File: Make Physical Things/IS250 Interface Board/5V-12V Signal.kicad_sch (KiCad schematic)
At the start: 5 parts, among them Q10 PN2222A, Q11 PN2907A

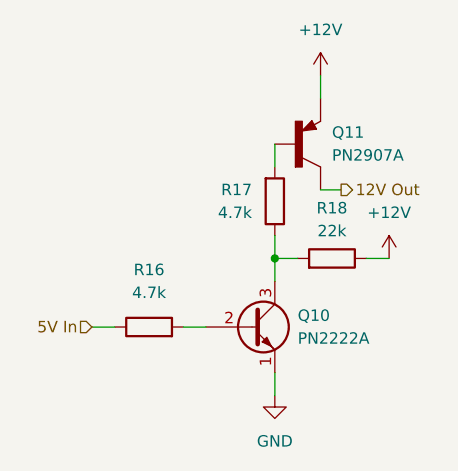
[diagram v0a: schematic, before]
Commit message: More PCB Layout
PCB laid out further, and just requires routing and silkscreen.
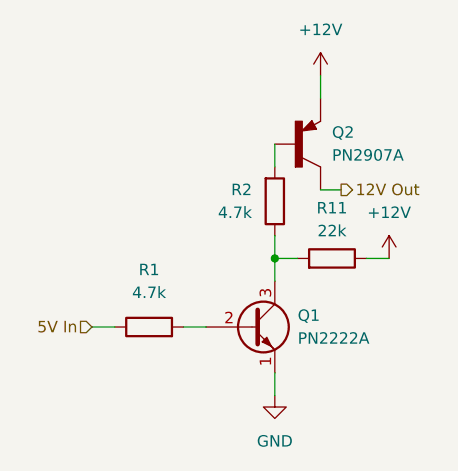
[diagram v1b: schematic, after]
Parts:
- renumbered Q10 to Q1, Q11 to Q2, R16 to R1, R18 to R11, R17 to R2
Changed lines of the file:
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@@
   (symbol (lib_id "Device:R") (at 77.47 88.9 270) (mirror x)
     (in_bom yes) (on_board yes)
-    (property "Reference" "R18" (id 0) (at 77.47 83.312 90))
+    (property "Reference" "R11" (id 0) (at 77.47 83.312 90))
     (property "Value" "22k" (id 1) (at 77.47 85.852 90))
     (property "Footprint" "Resistor_THT:R_Axial_DIN0207_L6.3mm_D2.5mm_P10.16mm_Horizontal" (id 2) (at 77.47 90.678 90)
@@
   (symbol (lib_id "Transistor_BJT:PN2222A") (at 68.58 96.52 0)
     (in_bom yes) (on_board yes) (fields_autoplaced)
-    (property "Reference" "Q10" (id 0) (at 73.66 95.2499 0)
+    (property "Reference" "Q1" (id 0) (at 73.66 95.2499 0)
       (effects (font (size 1.27 1.27)) (justify left))
     )
@@
   (symbol (lib_id "Device:R") (at 71.12 82.55 0) (mirror x)
     (in_bom yes) (on_board yes) (fields_autoplaced)
-    (property "Reference" "R17" (id 0) (at 68.58 81.2799 0)
+    (property "Reference" "R2" (id 0) (at 68.58 81.2799 0)
       (effects (font (size 1.27 1.27)) (justify right))
     )
@@
   (symbol (lib_id "PN2907A:PN2907A") (at 73.66 76.2 0)
     (in_bom yes) (on_board yes) (fields_autoplaced)
-    (property "Reference" "Q11" (id 0) (at 77.47 74.9045 0)
+    (property "Reference" "Q2" (id 0) (at 77.47 74.9045 0)
       (effects (font (size 1.27 1.27)) (justify left))
     )
@@
   (symbol (lib_id "Device:R") (at 57.15 96.52 90)
     (in_bom yes) (on_board yes) (fields_autoplaced)
-    (property "Reference" "R16" (id 0) (at 57.15 90.17 90))
+    (property "Reference" "R1" (id 0) (at 57.15 90.17 90))
     (property "Value" "4.7k" (id 1) (at 57.15 92.71 90))
     (property "Footprint" "Resistor_THT:R_Axial_DIN0207_L6.3mm_D2.5mm_P10.16mm_Horizontal" (id 2) (at 57.15 98.298 90)

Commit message: PCB Layout Finalised
Finalised the layout, routing and silkscreen still to be completed.
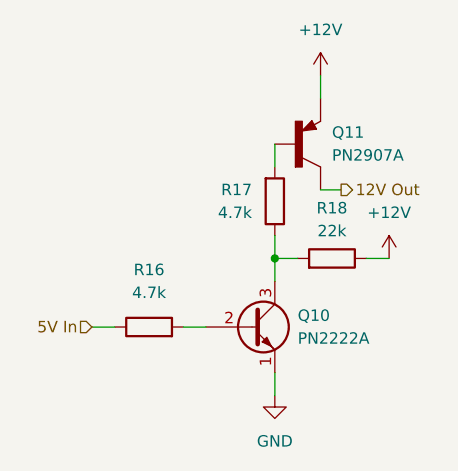
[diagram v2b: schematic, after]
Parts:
- renumbered Q1 to Q10, Q2 to Q11, R1 to R16, R2 to R17, R11 to R18
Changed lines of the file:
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@@
   (symbol (lib_id "Device:R") (at 77.47 88.9 270) (mirror x)
     (in_bom yes) (on_board yes)
-    (property "Reference" "R11" (id 0) (at 77.47 83.312 90))
+    (property "Reference" "R18" (id 0) (at 77.47 83.312 90))
     (property "Value" "22k" (id 1) (at 77.47 85.852 90))
     (property "Footprint" "Resistor_THT:R_Axial_DIN0207_L6.3mm_D2.5mm_P10.16mm_Horizontal" (id 2) (at 77.47 90.678 90)
@@
   (symbol (lib_id "Transistor_BJT:PN2222A") (at 68.58 96.52 0)
     (in_bom yes) (on_board yes) (fields_autoplaced)
-    (property "Reference" "Q1" (id 0) (at 73.66 95.2499 0)
+    (property "Reference" "Q10" (id 0) (at 73.66 95.2499 0)
       (effects (font (size 1.27 1.27)) (justify left))
     )
@@
   (symbol (lib_id "Device:R") (at 71.12 82.55 0) (mirror x)
     (in_bom yes) (on_board yes) (fields_autoplaced)
-    (property "Reference" "R2" (id 0) (at 68.58 81.2799 0)
+    (property "Reference" "R17" (id 0) (at 68.58 81.2799 0)
       (effects (font (size 1.27 1.27)) (justify right))
     )
@@
   (symbol (lib_id "PN2907A:PN2907A") (at 73.66 76.2 0)
     (in_bom yes) (on_board yes) (fields_autoplaced)
-    (property "Reference" "Q2" (id 0) (at 77.47 74.9045 0)
+    (property "Reference" "Q11" (id 0) (at 77.47 74.9045 0)
       (effects (font (size 1.27 1.27)) (justify left))
     )
@@
   (symbol (lib_id "Device:R") (at 57.15 96.52 90)
     (in_bom yes) (on_board yes) (fields_autoplaced)
-    (property "Reference" "R1" (id 0) (at 57.15 90.17 90))
+    (property "Reference" "R16" (id 0) (at 57.15 90.17 90))
     (property "Value" "4.7k" (id 1) (at 57.15 92.71 90))
     (property "Footprint" "Resistor_THT:R_Axial_DIN0207_L6.3mm_D2.5mm_P10.16mm_Horizontal" (id 2) (at 57.15 98.298 90)
